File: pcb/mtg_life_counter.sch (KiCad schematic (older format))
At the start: 97 parts, among them J1 USB C 4907, J2 ICSP, J3 TP_UART, SW1 SW_SPST, SW2 SW_SPST, U1 ATmega328P-AU, U2 74HC595, U3 74HC595, U4 74HC595, U5 74HC595, U6 TPIC6B595, U7 TPIC6B595, U8 74HC165, Y1 16MHz

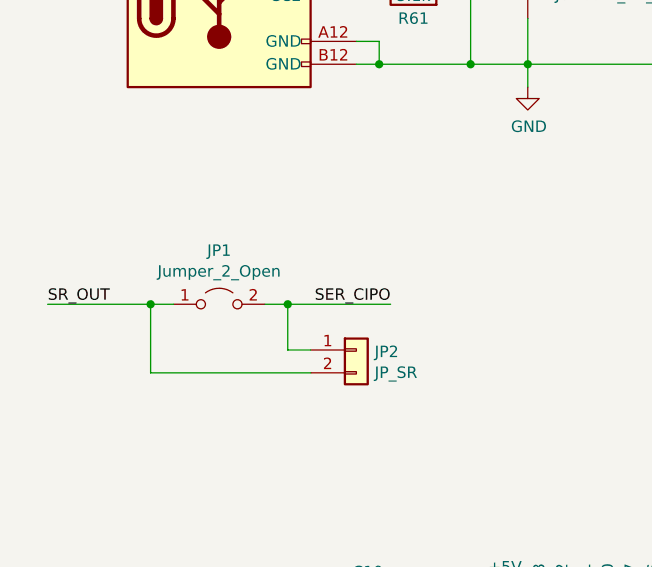
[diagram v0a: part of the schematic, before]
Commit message: Resolve design review issues
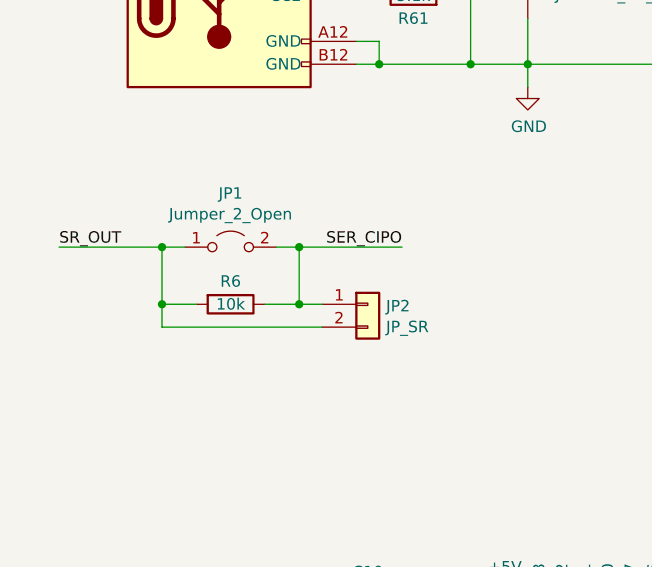
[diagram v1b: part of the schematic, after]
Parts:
- added R6: 10k, Resistor_SMD:R_0805_2012Metric_Pad1.15x1.40mm_HandSolder, symbol Device:R
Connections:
- net SER_CIPO: now also R6.1
- net SR_OUT: now also R6.2
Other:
- moved on the sheet: JP1, JP2
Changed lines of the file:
@@
 L Jumper:Jumper_2_Open JP1
 U 1 1 61C0859C
-P 1750 6750
-F 0 "JP1" H 1750 6985 50  0000 C CNN
-F 1 "Jumper_2_Open" H 1750 6894 50  0000 C CNN
-F 2 "Jumper:SolderJumper-2_P1.3mm_Open_TrianglePad1.0x1.5mm" H 1750 6750 50  0001 C CNN
-F 3 "~" H 1750 6750 50  0001 C CNN
-	1    1750 6750
+P 1800 6500
+F 0 "JP1" H 1800 6735 50  0000 C CNN
+F 1 "Jumper_2_Open" H 1800 6644 50  0000 C CNN
+F 2 "Jumper:SolderJumper-2_P1.3mm_Open_TrianglePad1.0x1.5mm" H 1800 6500 50  0001 C CNN
+F 3 "~" H 1800 6500 50  0001 C CNN
+	1    1800 6500
 	1    0    0    -1
 $EndComp
@@
 Wire Wire Line
 	1600 8550 2100 8550
-Text Label 1000 6750 0    50   ~ 0
+Text Label 1050 6500 0    50   ~ 0
 SR_OUT
-Text Label 2500 6750 2    50   ~ 0
+Text Label 2550 6500 2    50   ~ 0
 SER_CIPO
 Wire Wire Line
-	1550 6750 1450 6750
+	1600 6500 1500 6500
 Wire Wire Line
 	2000 9250 2000 9550
@@
 	6500 4850 6250 4850
 Wire Wire Line
-	1950 6750 2050 6750
+	2000 6500 2100 6500
 $Comp
 L power:+5V #PWR0136
@@
 L Connector_Generic:Conn_01x02 JP2
 U 1 1 6304655D
-P 2350 6950
-F 0 "JP2" H 2430 6942 50  0000 L CNN
-F 1 "JP_SR" H 2430 6851 50  0000 L CNN
-F 2 "mtg_life_counter:TP_Edge_2" H 2350 6950 50  0001 C CNN
-F 3 "~" H 2350 6950 50  0001 C CNN
-	1    2350 6950
-	1    0    0    -1
-$EndComp
-Wire Wire Line
-	2050 6750 2050 6950
-Wire Wire Line
-	2050 6950 2150 6950
-Connection ~ 2050 6750
-Wire Wire Line
-	2050 6750 2500 6750
-Wire Wire Line
-	1450 6750 1450 7050
-Wire Wire Line
-	1450 7050 2150 7050
-Connection ~ 1450 6750
-Wire Wire Line
-	1450 6750 1000 6750
+P 2400 6750
+F 0 "JP2" H 2480 6742 50  0000 L CNN
+F 1 "JP_SR" H 2480 6651 50  0000 L CNN
+F 2 "mtg_life_counter:TP_Edge_2" H 2400 6750 50  0001 C CNN
+F 3 "~" H 2400 6750 50  0001 C CNN
+	1    2400 6750
+	1    0    0    -1
+$EndComp
+Connection ~ 2100 6500
+Wire Wire Line
+	2100 6500 2550 6500
+Wire Wire Line
+	1500 6500 1500 6750
+Wire Wire Line
+	1500 6850 2200 6850
+Connection ~ 1500 6500
+Wire Wire Line
+	1500 6500 1050 6500
 Wire Wire Line
 	3550 8450 3550 8950
@@
 $EndComp
 $Comp
-L power:+5V #PWR?
+L power:+5V #PWR0139
 U 1 1 63669CBE
 P 6300 2550
-F 0 "#PWR?" H 6300 2400 50  0001 C CNN
+F 0 "#PWR0139" H 6300 2400 50  0001 C CNN
 F 1 "+5V" H 6315 2723 50  0000 C CNN
 F 2 "" H 6300 2550 50  0001 C CNN
@@
 Wire Wire Line
 	6300 2550 6700 2550
+$Comp
+L Device:R R6
+U 1 1 63888C60
+P 1800 6750
+F 0 "R6" V 1700 6750 50  0000 C CNN
+F 1 "10k" V 1800 6750 50  0000 C CNN
+F 2 "Resistor_SMD:R_0805_2012Metric_Pad1.15x1.40mm_HandSolder" V 1730 6750 50  0001 C CNN
+F 3 "~" H 1800 6750 50  0001 C CNN
+	1    1800 6750
+	0    1    1    0
+$EndComp
+Wire Wire Line
+	1650 6750 1500 6750
+Connection ~ 1500 6750
+Wire Wire Line
+	1950 6750 2100 6750
+Wire Wire Line
+	2100 6500 2100 6750
+Connection ~ 2100 6750
+Wire Wire Line
+	2100 6750 2200 6750
+Wire Wire Line
+	1500 6750 1500 6850
 $EndSCHEMATC
